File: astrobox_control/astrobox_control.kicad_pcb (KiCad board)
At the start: 2 copper layers, 153 x 133 mm, 229 parts, among them J1 INTERCOM2, J10 OUT_CARPLUG, J13 OUT_12V_1, J15 OUT_12V_2, J17 OUT_12V_3, J18 OUT_6V_1, J2 HEAT_SEC, J20 OUT_6V_2, J22 OUT_6V_3, J24 OUT_5V_1, J26 OUT_5V_2, J28 OUT_5V_3, J3 HEAT_SCOPE, J30 OUT_9V_1, J32 OUT_9V_2, J34 OUT_9V_3, J4 HEAD_EYE, J5 FANS, J6 Fader_PWM1, J7 Fader_PWM2, J8 Fader_PWM3, J9 ISP_PWM_Driver, Q1 BC327, Q10 IRLZ34N, Q11 IRLZ34N, Q12 IRLZ34N, Q13 IRLZ34N, Q14 IRLZ34N, Q15 IRLZ34N, Q16 IRLZ34N, Q17 IRLZ34N, Q18 IRLZ34N, Q19 IRLZ34N, Q2 IRLZ34N, Q20 IRLZ34N, Q21 IRLZ34N, Q3 BC327, Q4 IRLZ34N, Q5 BC327, Q6 IRLZ34N, Q7 BC327, Q8 IRLZ34N, Q9 IRLZ34N, SW1 PWM1_ON, SW10 PRESET4, SW11 PRESET5, SW12 PWM3_AUTOHUM, SW13 PRESET6, SW14 PRESETW, SW15 PWR_OUT_CARPLUG, SW16 PWR_OUT_12V_1, SW17 PWR_OUT_12V_2, SW18 PWR_OUT_12V_3, SW19 PWR_OUT_6V_1, SW2 PWM2_ON, SW20 PWR_OUT_6V_2, SW21 PWR_OUT_6V_3, SW22 PWR_OUT_5V_1, SW23 PWR_OUT_5V_2, SW24 PWR_OUT_5V_3, SW25 PWR_OUT_9V_1, SW26 PWR_OUT_9V_2, SW27 PWR_OUT_9V_3, SW3 PWM3_ON, SW4 PWM4_ON, SW5 PRESET1, SW6 PWM1_AUTOHUM, SW7 PRESET2, SW8 PRESET3, SW9 PWM2_AUTOHUM, U1 L78S10, U10 L7806CV, U11 L7806CV, U12 L7806CV, U13 LM7805, U14 LM7805, U15 LM7805, U16 LM7809, U17 LM7809, U18 LM7809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

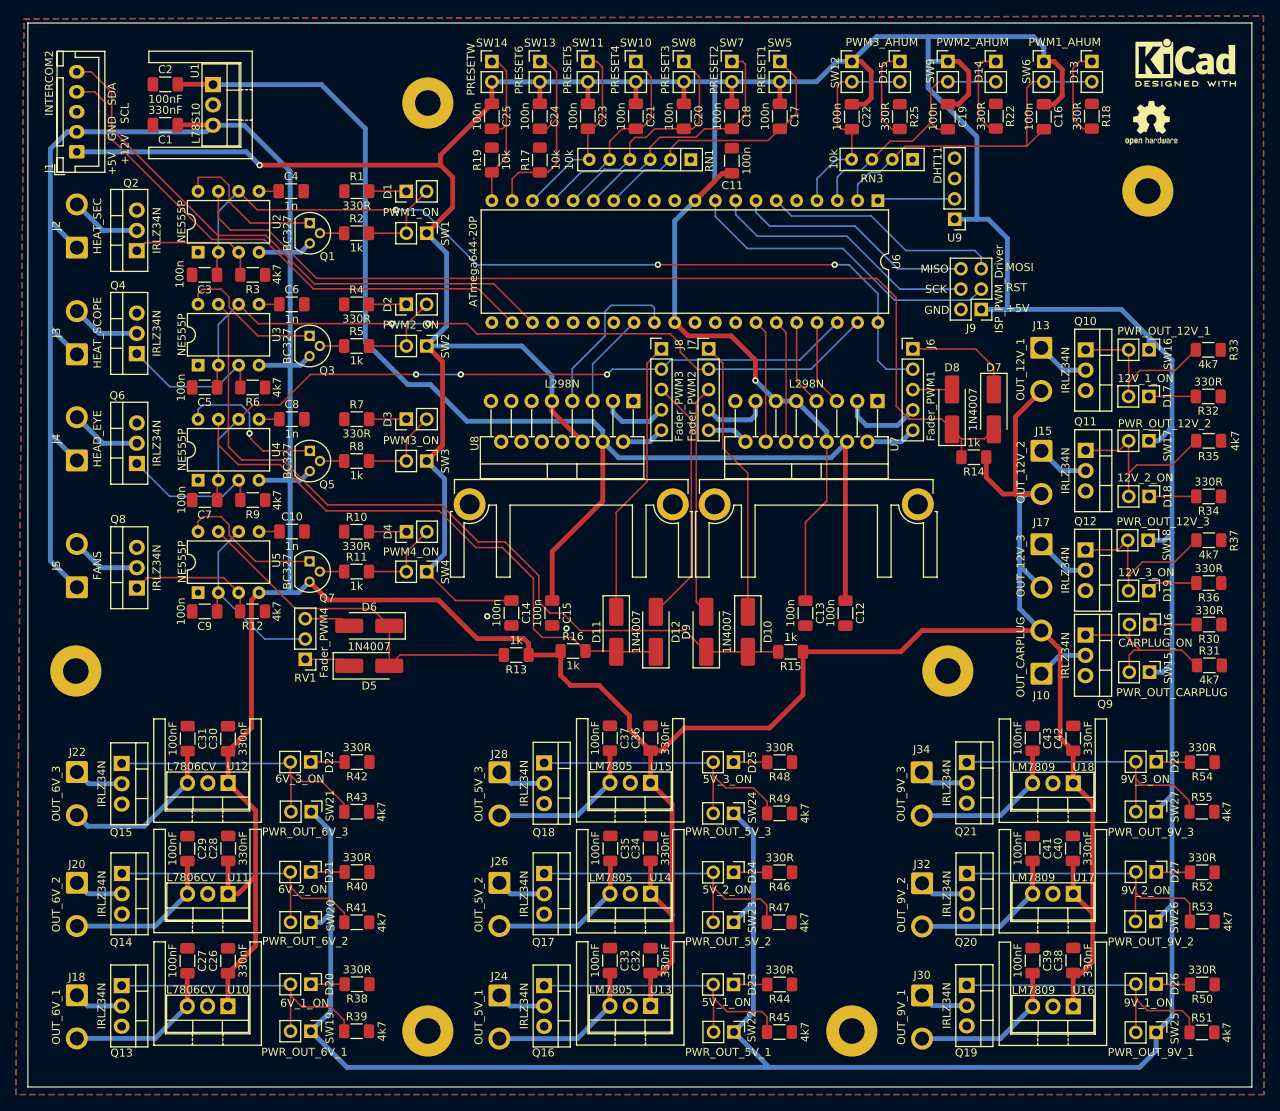
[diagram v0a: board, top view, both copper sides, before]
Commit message: astrobox WIP
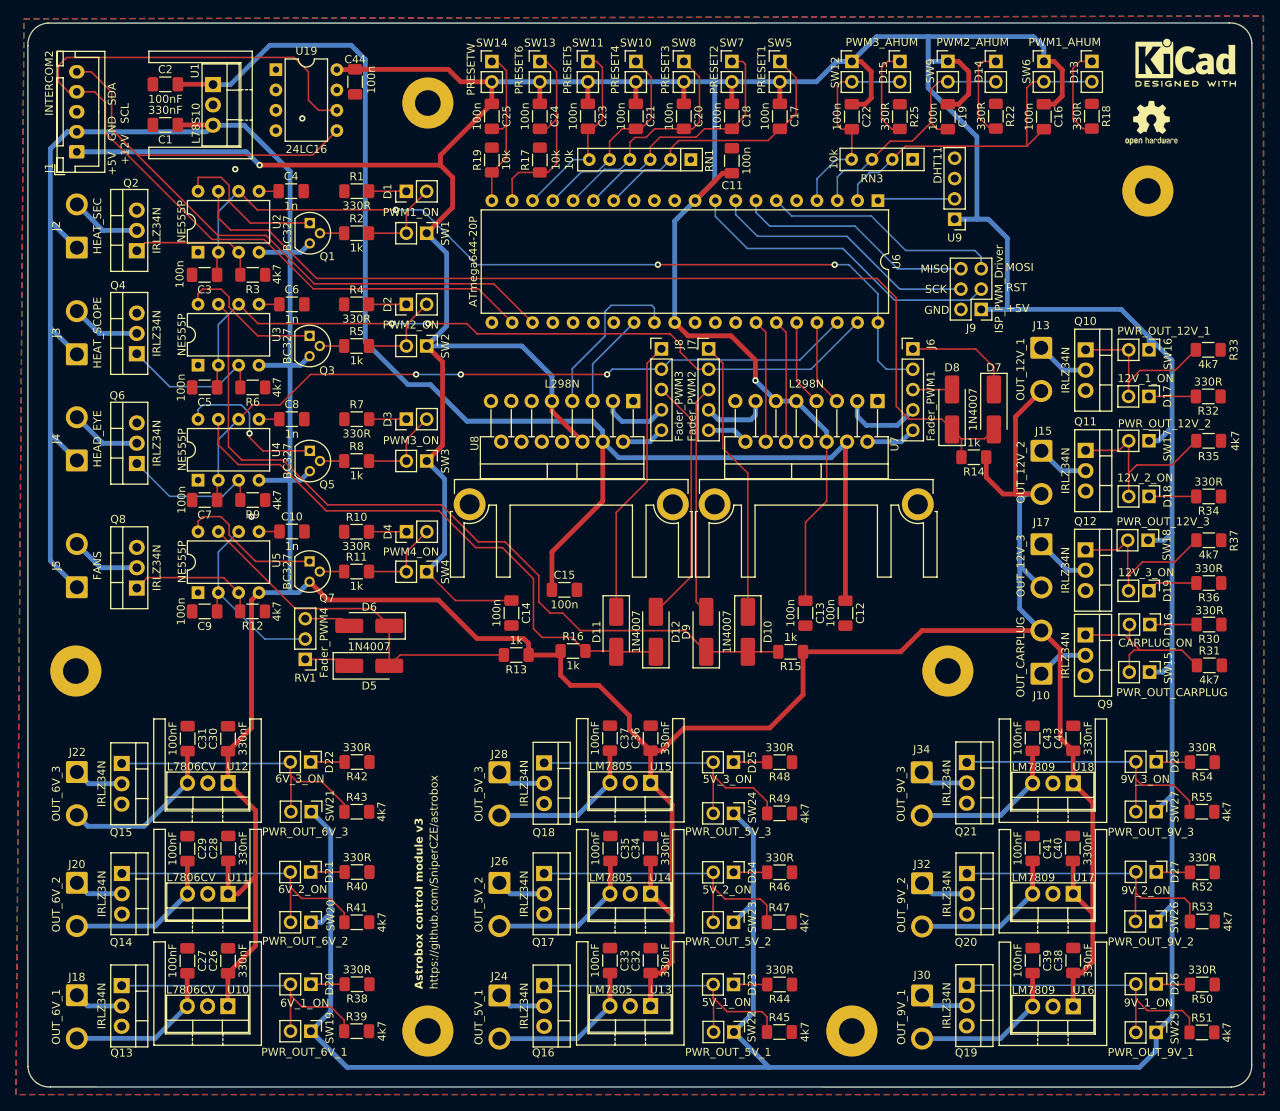
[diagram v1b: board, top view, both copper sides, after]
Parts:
- added C44: 100n, Capacitor_SMD:C_1206_3216Metric_Pad1.33x1.80mm_HandSolder, F.Cu at (57.9, 22.4)
- added U19: 24LC16, Package_DIP:DIP-8_W7.62mm, F.Cu at (48.0, 20.8)
- moved C15 3.27 mm to (84.1, 85.9), turned to 0 degrees
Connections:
- REF** pad 1: (no net) -> GND
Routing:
- net /PWM control plane/SCL: track 68.6 -> 113.5 mm
- net /PWM control plane/SDA: track 72.7 -> 98.8 mm
- net +5V: track 717.4 -> 735.5 mm
- net +10V: track 162.6 -> 170.1 mm
- net +12V: track 517.7 -> 516.6 mm
- net /PWM control plane/PRESET5: track 24.1 -> 23.2 mm
- net Net-(D14-K): track 11.5 -> 10.8 mm
- net /PWM control plane/PRESETW: track 21.3 -> 20.6 mm
- net Net-(D28-A): track 36.6 -> 36.0 mm
- net /PWM control plane/PRESET4: track 25.8 -> 25.2 mm
- net GND: vias 2 -> 3
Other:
- outline, holes or cut-outs redrawn
- board text added: "Astrobox control module v3"
- board text added: "https://github.com/SniperCZE/astrobox"
